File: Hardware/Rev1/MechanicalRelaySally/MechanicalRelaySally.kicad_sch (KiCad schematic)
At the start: 0 parts

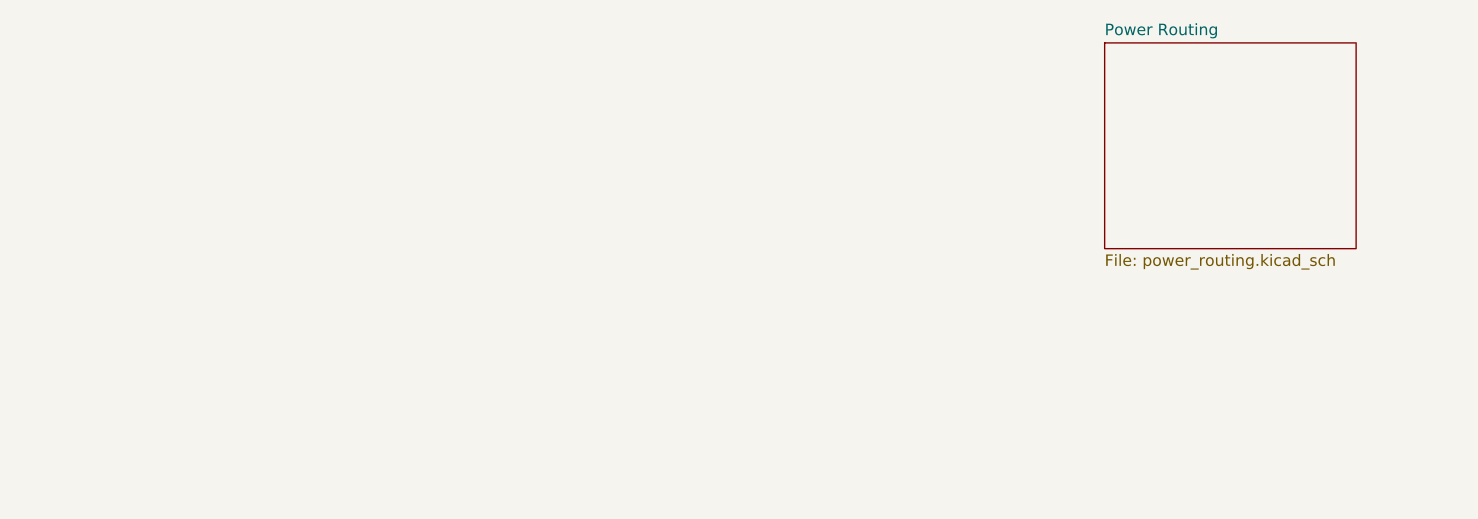
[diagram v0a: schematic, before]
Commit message: A
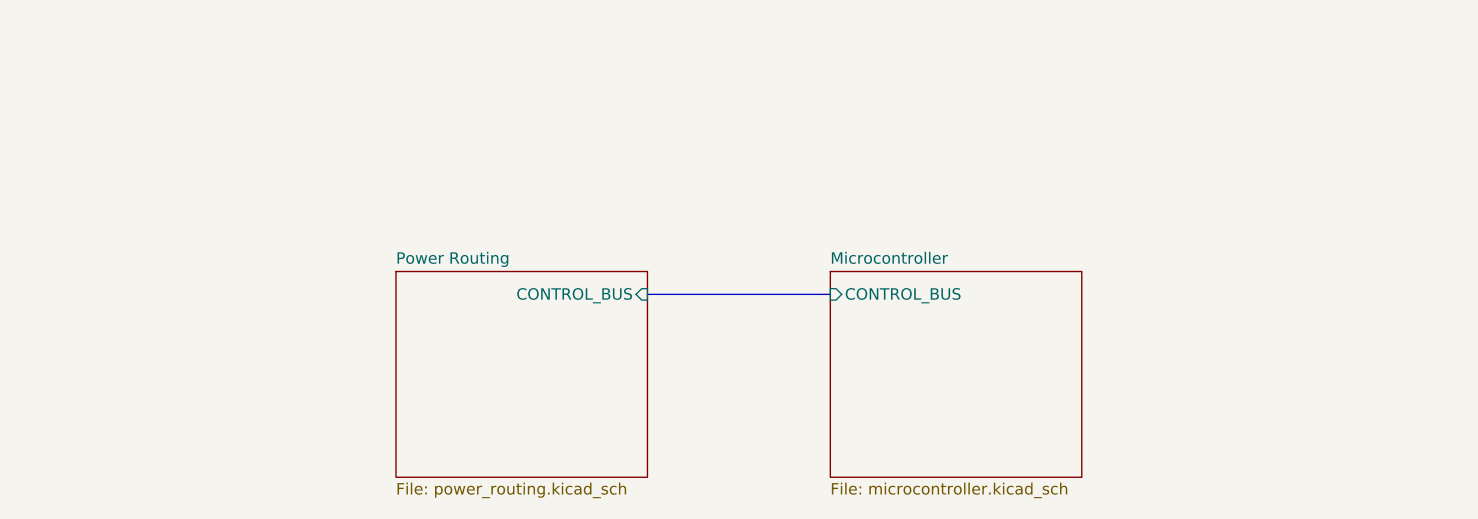
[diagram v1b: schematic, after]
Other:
- added sheet Microcontroller (microcontroller.kicad_sch)
- sheet Power Routing ports: added CONTROL_BUS; removed none
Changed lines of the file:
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@@
 	(generator_version "9.0")
 	(paper "A4")
+	(bus
+		(pts
+			(xy 81.28 53.34) (xy 101.6 53.34)
+		)
+		(stroke
+			(width 0)
+			(type default)
+		)
+	)
 	(sheet
-		(at 132.08 25.4)
+		(at 53.34 50.8)
 		(size 27.94 22.86)
 		(exclude_from_sim no)
@@
 		)
 		(property "Sheetname" "Power Routing"
-			(at 132.08 24.6884 0)
+			(at 53.34 50.0884 0)
 			(effects
 				(font
@@
 		)
 		(property "Sheetfile" "power_routing.kicad_sch"
-			(at 132.08 48.8446 0)
+			(at 53.34 74.2446 0)
 			(effects
 				(font
@@
 				)
 				(justify left top)
+			)
+		)
+		(pin "CONTROL_BUS" input
+			(at 81.28 53.34 0)
+			(effects
+				(font
+					(size 1.27 1.27)
+				)
+				(justify right)
 			)
 		)
@@
 				)
 			)
+		)
+	)
+	(sheet
+		(at 101.6 50.8)
+		(size 27.94 22.86)
+		(exclude_from_sim no)
+		(in_bom yes)
+		(on_board yes)
+		(dnp no)
+		(fields_autoplaced yes)
+		(stroke
+			(width 0.1524)
+			(type solid)
+		)
+		(fill
+			(color 255 255 194 1.0000)
+		)
+		(property "Sheetname" "Microcontroller"
+			(at 101.6 50.0884 0)
+			(effects
+				(font
+					(size 1.27 1.27)
+				)
+				(justify left bottom)
+			)
+		)
+		(property "Sheetfile" "microcontroller.kicad_sch"
+			(at 101.6 74.2446 0)
+			(effects
+				(font
+					(size 1.27 1.27)
+				)
+				(justify left top)
+			)
+		)
+		(pin "CONTROL_BUS" input
+			(at 101.6 53.34 180)
+			(effects
+				(font
+					(size 1.27 1.27)
+				)
+				(justify left)
+			)
+		)
+		(instances
+			(project "MechanicalRelaySally"
+				(path "/fc3bfb83-1db4-4bd1-b480-85f699496fec"
+					(page "8")
+				)
+			)

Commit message: A
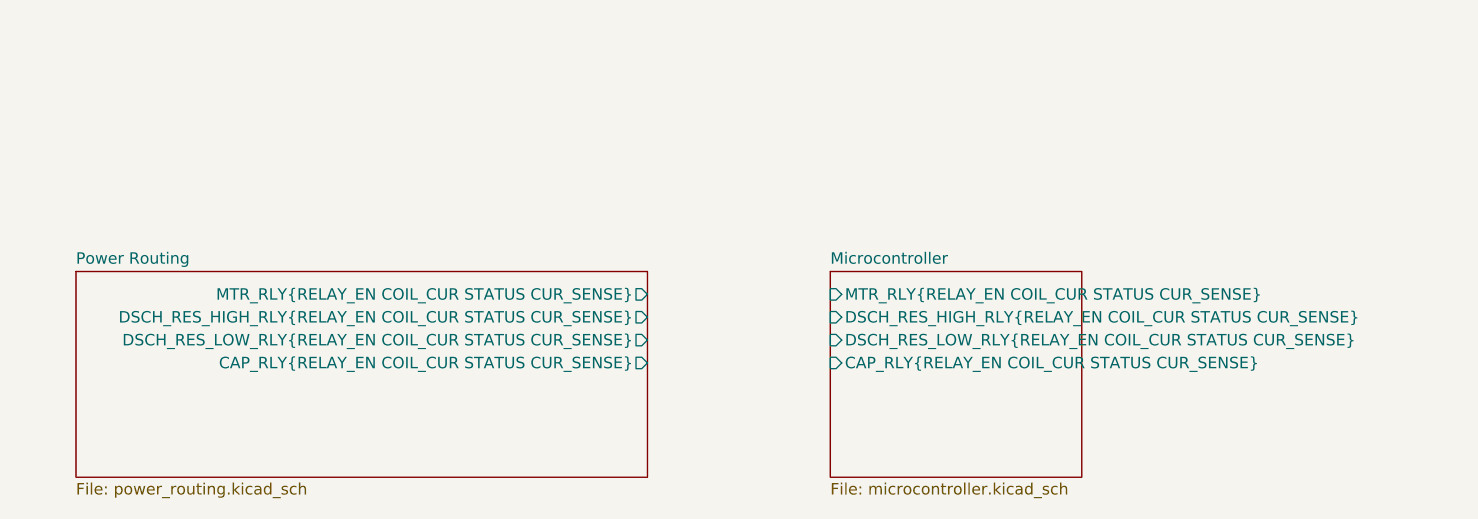
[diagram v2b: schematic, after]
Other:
- sheet Microcontroller ports: added CAP_RLY{RELAY_EN COIL_CUR STATUS CUR_SENSE}, DSCH_RES_HIGH_RLY{RELAY_EN COIL_CUR STATUS CUR_SENSE}, DSCH_RES_LOW_RLY{RELAY_EN COIL_CUR STATUS CUR_SENSE}, MTR_RLY{RELAY_EN COIL_CUR STATUS CUR_SENSE}; removed CONTROL_BUS
- sheet Power Routing ports: added CAP_RLY{RELAY_EN COIL_CUR STATUS CUR_SENSE}, DSCH_RES_HIGH_RLY{RELAY_EN COIL_CUR STATUS CUR_SENSE}, DSCH_RES_LOW_RLY{RELAY_EN COIL_CUR STATUS CUR_SENSE}, MTR_RLY{RELAY_EN COIL_CUR STATUS CUR_SENSE}; removed CONTROL_BUS
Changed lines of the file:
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@@
 	(generator_version "9.0")
 	(paper "A4")
-	(bus
-		(pts
-			(xy 81.28 53.34) (xy 101.6 53.34)
-		)
-		(stroke
-			(width 0)
-			(type default)
-		)
-	)
 	(sheet
-		(at 53.34 50.8)
-		(size 27.94 22.86)
+		(at 17.78 50.8)
+		(size 63.5 22.86)
 		(exclude_from_sim no)
 		(in_bom yes)
@@
 		)
 		(property "Sheetname" "Power Routing"
-			(at 53.34 50.0884 0)
+			(at 17.78 50.0884 0)
 			(effects
 				(font
@@
 		)
 		(property "Sheetfile" "power_routing.kicad_sch"
-			(at 53.34 74.2446 0)
+			(at 17.78 74.2446 0)
 			(effects
 				(font
@@
 			)
 		)
-		(pin "CONTROL_BUS" input
+		(pin "MTR_RLY{RELAY_EN COIL_CUR STATUS CUR_SENSE}" output
 			(at 81.28 53.34 0)
+			(effects
+				(font
+					(size 1.27 1.27)
+				)
+				(justify right)
+			)
+		)
+		(pin "DSCH_RES_HIGH_RLY{RELAY_EN COIL_CUR STATUS CUR_SENSE}" output
+			(at 81.28 55.88 0)
+			(effects
+				(font
+					(size 1.27 1.27)
+				)
+				(justify right)
+			)
+		)
+		(pin "DSCH_RES_LOW_RLY{RELAY_EN COIL_CUR STATUS CUR_SENSE}" output
+			(at 81.28 58.42 0)
+			(effects
+				(font
+					(size 1.27 1.27)
+				)
+				(justify right)
+			)
+		)
+		(pin "CAP_RLY{RELAY_EN COIL_CUR STATUS CUR_SENSE}" output
+			(at 81.28 60.96 0)
 			(effects
 				(font
@@
 			)
 		)
-		(pin "CONTROL_BUS" input
+		(pin "CAP_RLY{RELAY_EN COIL_CUR STATUS CUR_SENSE}" input
+			(at 101.6 60.96 180)
+			(effects
+				(font
+					(size 1.27 1.27)
+				)
+				(justify left)
+			)
+		)
+		(pin "DSCH_RES_HIGH_RLY{RELAY_EN COIL_CUR STATUS CUR_SENSE}" input
+			(at 101.6 55.88 180)
+			(effects
+				(font
+					(size 1.27 1.27)
+				)
+				(justify left)
+			)
+		)
+		(pin "DSCH_RES_LOW_RLY{RELAY_EN COIL_CUR STATUS CUR_SENSE}" input
+			(at 101.6 58.42 180)
+			(effects
+				(font
+					(size 1.27 1.27)
+				)
+				(justify left)
+			)
+		)
+		(pin "MTR_RLY{RELAY_EN COIL_CUR STATUS CUR_SENSE}" input
 			(at 101.6 53.34 180)
 			(effects
